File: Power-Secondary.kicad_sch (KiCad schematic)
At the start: 34 parts, among them J1 SUPP PWR MON, J2 SUPP PWR 1, J3 SUPP PWR 2, J4 DCDC SUPPLY, J5 FUSE +12V, Q1 S1G1D2S2G2D1, Q1A1 SUP90P06, Q1A2 SUP90P06, Q1A3 SUP90P06, Q1A4 SUP90P06, Q2 S1G1D2S2G2D1, Q3 S1G1D2S2G2D1

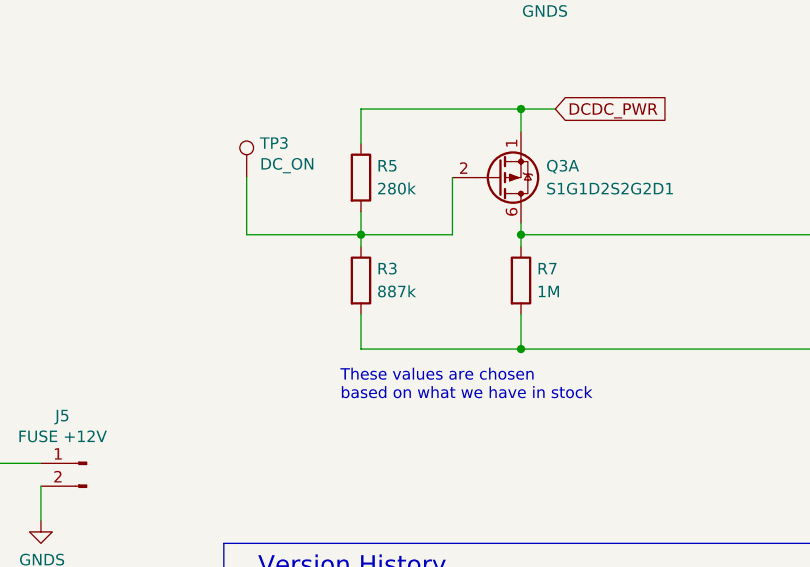
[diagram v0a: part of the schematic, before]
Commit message: Updated datasheets
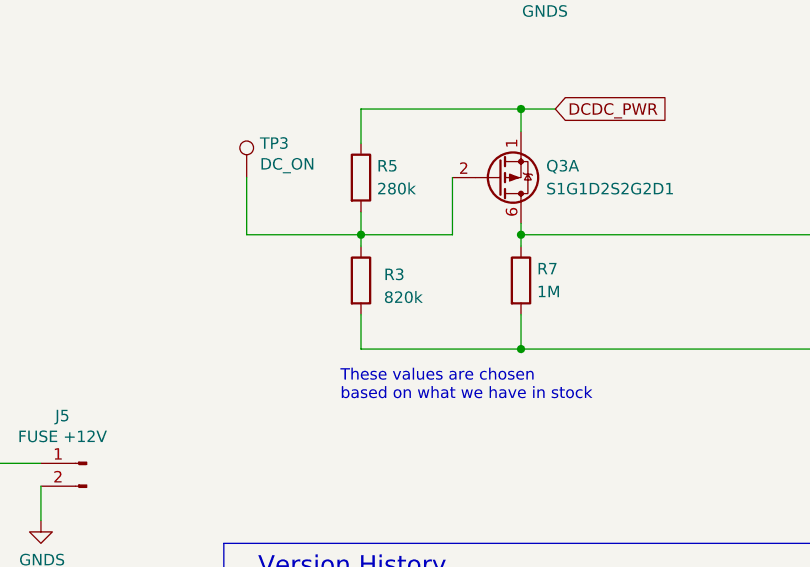
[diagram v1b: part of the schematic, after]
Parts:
- Q1A1, Q1A2, Q1A3, Q1A4: Manufacturer_Name Infineon -> (none); Manufacturer_Part_Number AUIRF4905 -> (none); Mouser Part Number 942-AUIRF4905 -> (none); Mouser Price/Stock https://www.mouser.co.uk/ProductDetail/Infineon-Technologie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 -> (none)
- R3: value 887k -> 820k
